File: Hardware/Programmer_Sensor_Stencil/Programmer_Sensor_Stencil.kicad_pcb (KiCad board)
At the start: 2 copper layers, 85 x 38.8 mm, 152 parts, among them J101 IDC Connector, J102 PicoBlade, J103 USB_C_USB2.0, J301 TC2030-NL, J302 PicoBlade, J501 RJ45_Input, J502 RJ45_Output, SW301 Reset, SW501 Slide Switch, U1 TPD4E02B04, U101 TPS25942ARVCR, U102 TPS7A20L_3V3, U103 USBLC6-2SC6, U201 FT2232HQ, U201 TPS7A20L_1V2, U202 93LC56B, U202 TPS7A20L_2V2, U203 TPS7A20L_3V3, U204 TLV840, U301 ICE40UL1K-CM36AI, U302 TPD4E02B04, U305 N25Q032A, U401 BNO086, U501 TPD4E02B04, U502 TPD4E02B04, U503 TPD4E02B04, U504 TPD4E02B04, U505 CBTU02044, Y201 16MHz, Y301 ASCO, Y401 32.768 kHz

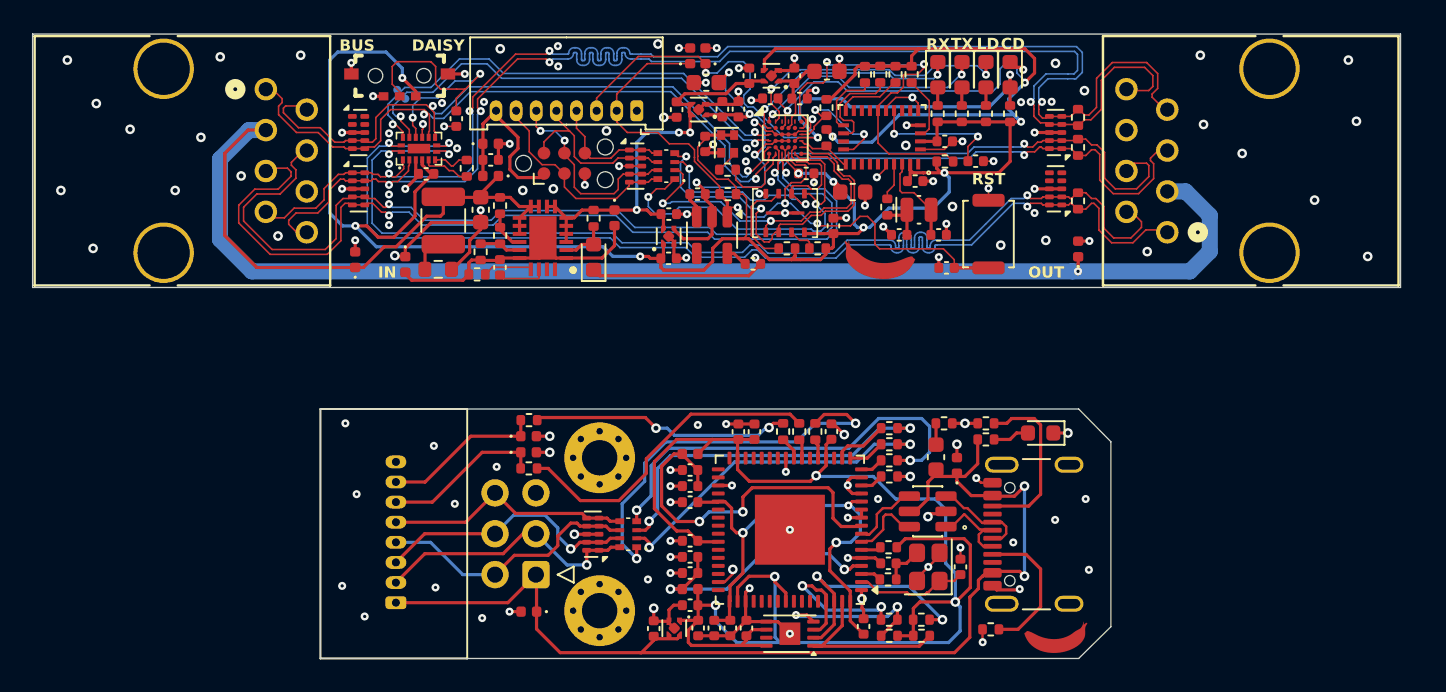
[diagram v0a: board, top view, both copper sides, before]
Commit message: Commited the final manufacturing files, as well as updated the documentation
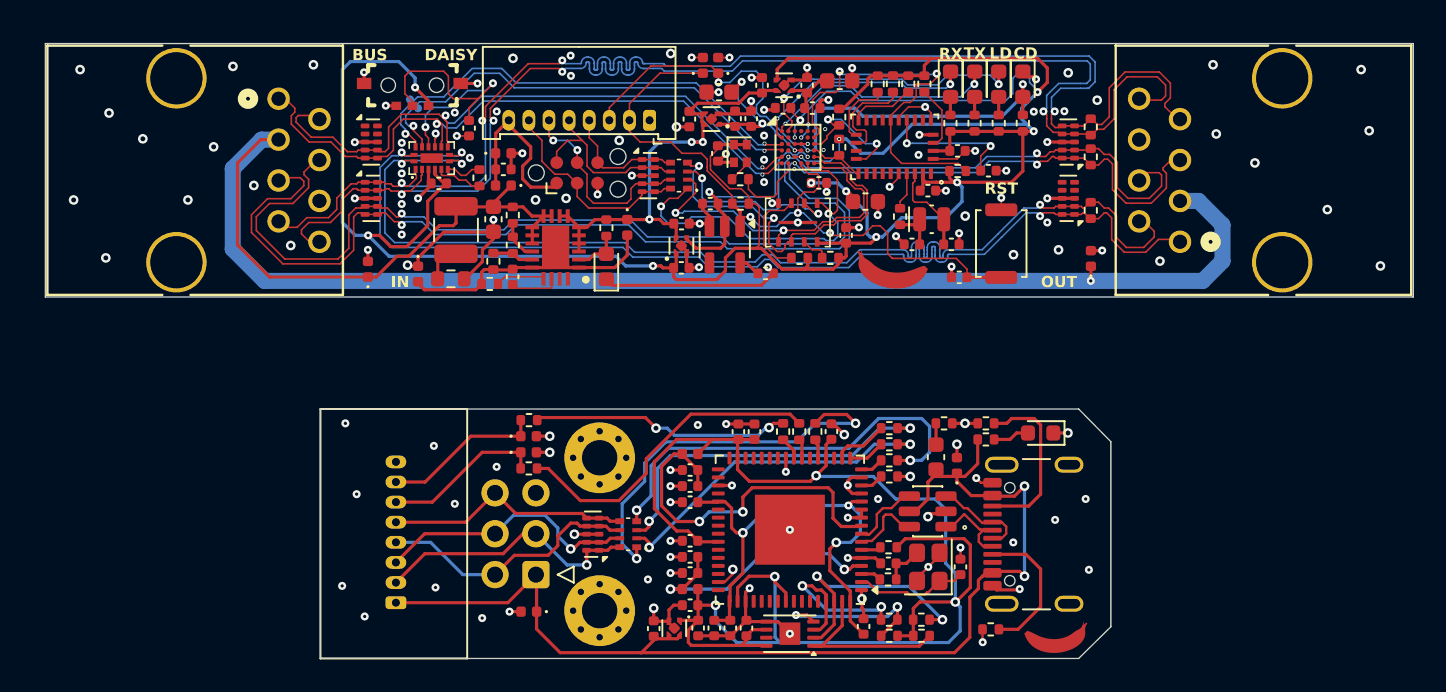
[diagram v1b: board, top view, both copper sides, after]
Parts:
- U301: footprint Custom_VoxLink_Footprints:ICE40UL1K_UCBGA-36 -> Package_BGA:UCBGA-36_2.5x2.5mm_Layout6x6_P0.4mm
- moved C101 0.99 mm to (139.4, 81.8)
- moved C102 0.99 mm to (141.7, 81.1)
- moved C103 0.99 mm to (142.9, 84.7)
- moved C201 0.99 mm to (153.9, 74.9)
- moved C202 0.99 mm to (156.8, 74.9)
- moved C207 0.99 mm to (155.2, 80.1)
- moved C208 0.99 mm to (158.7, 84.5)
- moved C210 0.99 mm to (157.8, 74.9)
- moved C213 0.99 mm to (163.2, 72.5)
- moved C214 0.99 mm to (161.6, 74.2)
- moved C215 0.99 mm to (164.8, 80.0)
- moved C301 0.99 mm to (142.4, 78.0)
- moved C302 0.99 mm to (163.7, 82.1)
- moved C304 0.99 mm to (170.7, 84.7)
- moved C401 0.99 mm to (168.7, 79.3)
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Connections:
- U301 pad C2: GND -> unconnected-(U301C-IOT_27A-PadC2)
- U301 pad D2: +1V2_CORE -> unconnected-(U301B-IOB_8A_G4-PadD2)
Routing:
- net GND: track 130.2 -> 126.4 mm, vias 143 -> 145
- net /System/CDONE: track 41.1 -> 38.3 mm
- net /Connectivity/VOX_RX_N: track 41.8 -> 39.8 mm
- net /Connectivity/VOX_RX_P: track 42.4 -> 40.4 mm
- net +3V3: track 273.9 -> 275.8 mm, vias 15 -> 17
- net +1V2_CORE: track 25.7 -> 24.7 mm
- net /System/FLASH_MISO: track 17.8 -> 16.8 mm, vias 2 -> 3
- net +2V5_NVCM: track 6.01 -> 6.02 mm, vias 0 -> 2
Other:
- board size 85 x 38.8 mm -> 85 x 38.2 mm
